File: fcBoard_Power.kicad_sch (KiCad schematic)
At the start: 24 parts, among them J1 DC_12V, U1 LM2596S-5, U2 LM2596S-ADJ, U3 LM2596S-ADJ

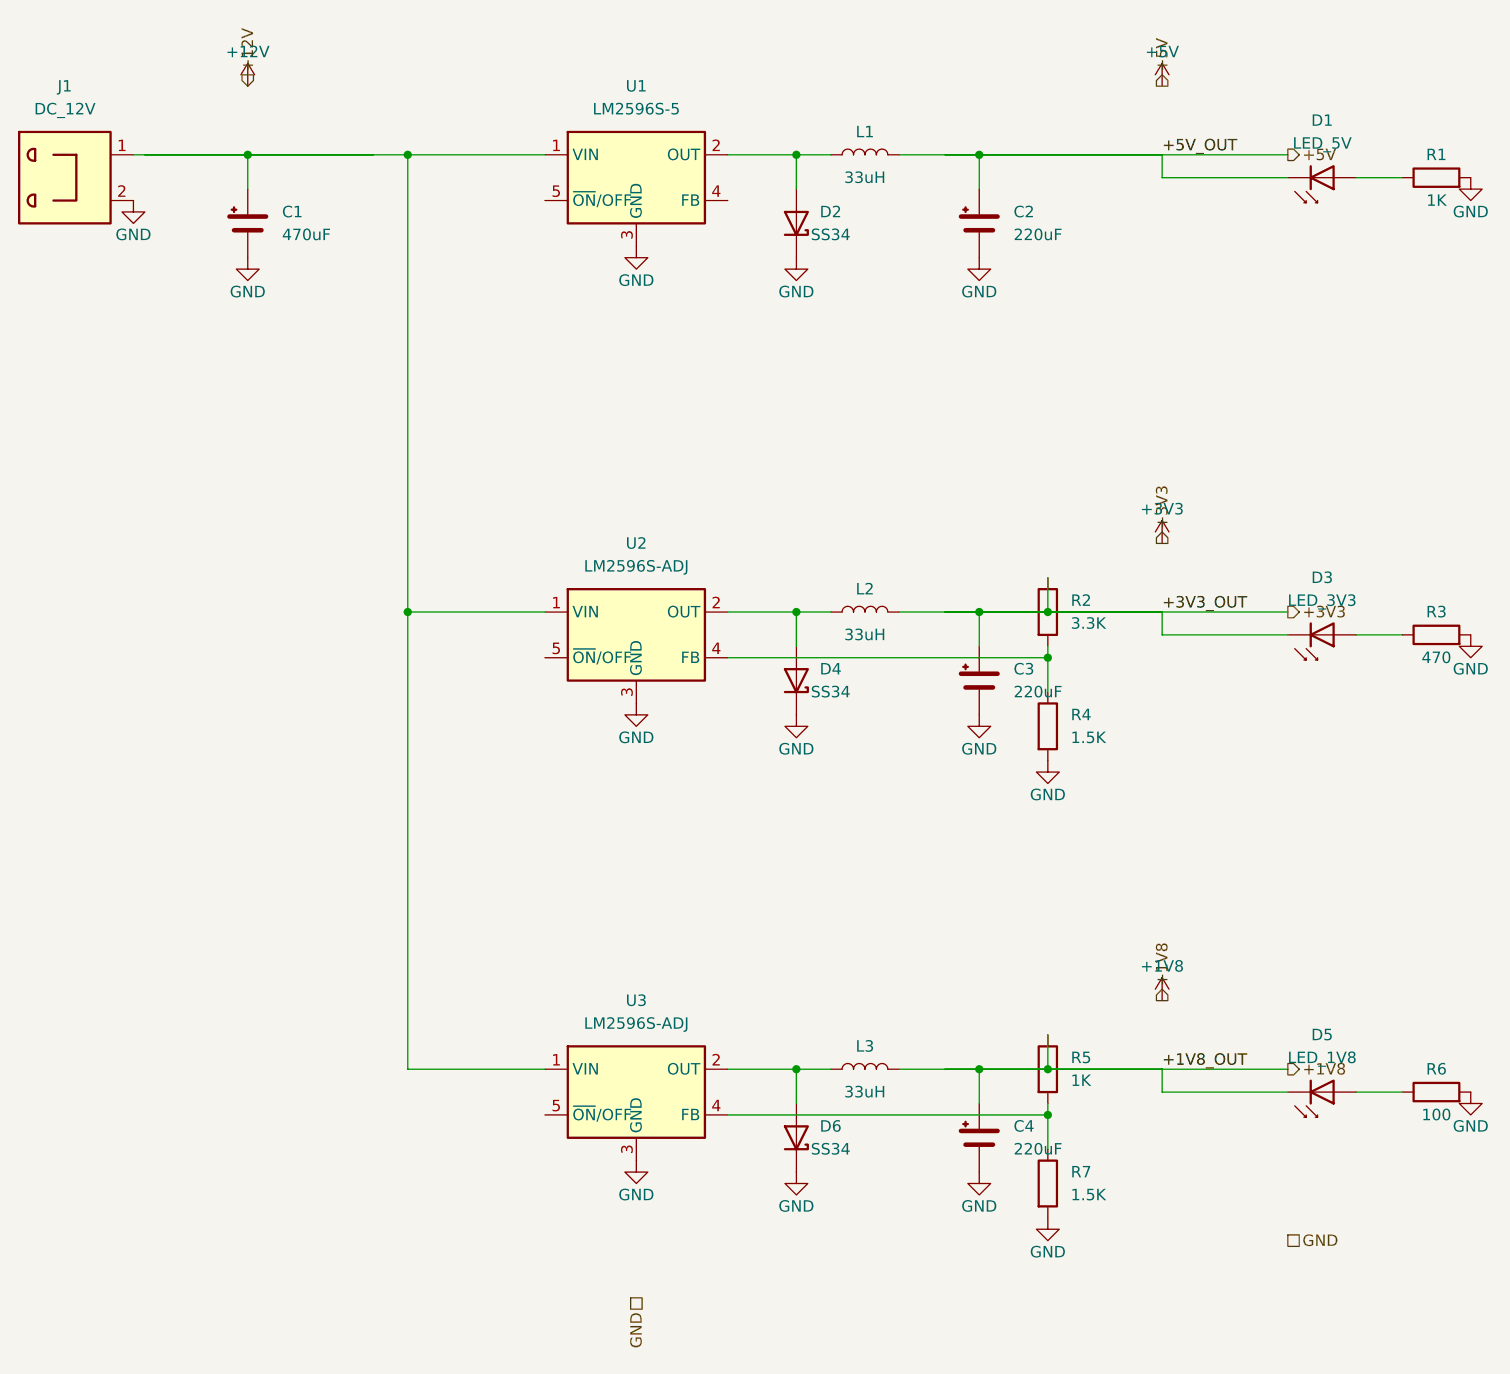
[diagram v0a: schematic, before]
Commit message: 회로도 라벨
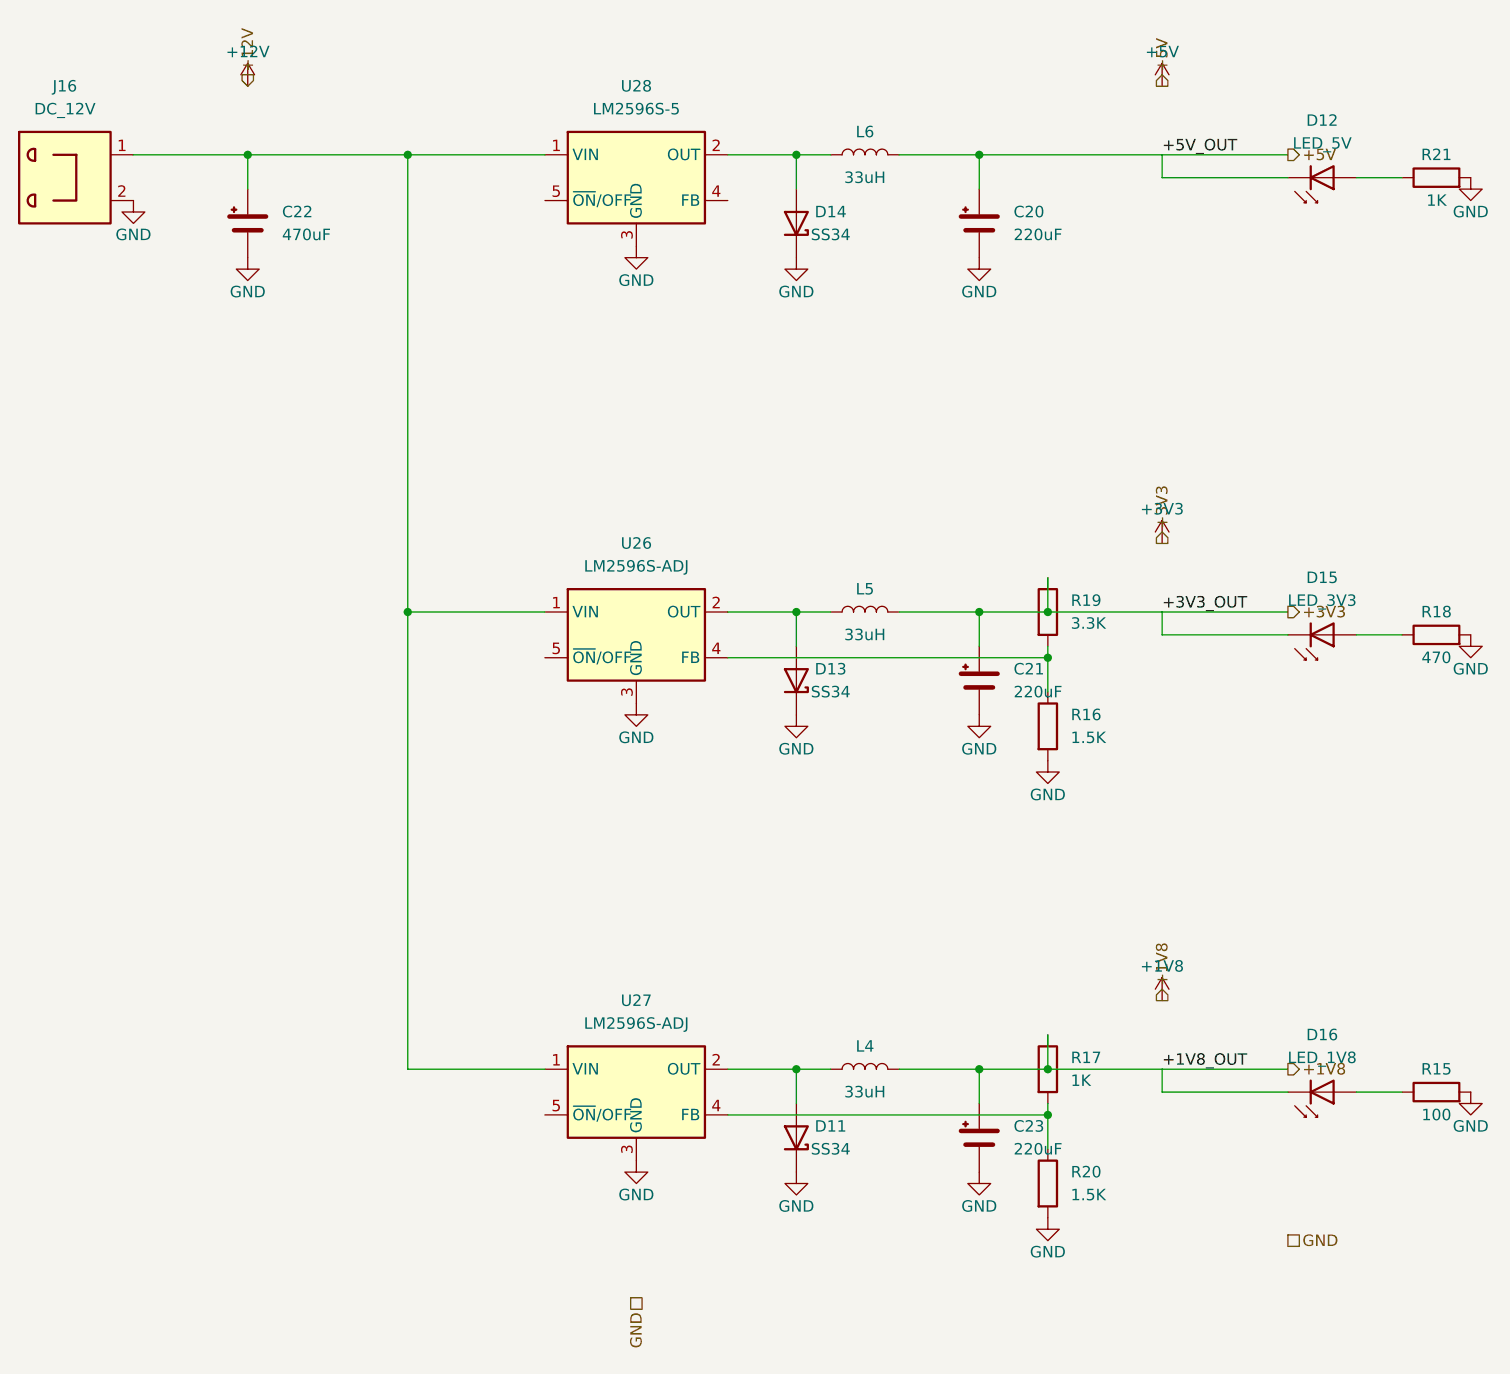
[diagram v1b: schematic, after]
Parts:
- renumbered C2 to C20, C3 to C21, C1 to C22, C4 to C23, D6 to D11, D1 to D12, D4 to D13, D2 to D14, D3 to D15, D5 to D16, J1 to J16, L3 to L4, L2 to L5, L1 to L6, R6 to R15, R4 to R16, R5 to R17, R3 to R18, R2 to R19, R7 to R20, R1 to R21, U2 to U26, U3 to U27, U1 to U28
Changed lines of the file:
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@@
 	(wire
 		(pts
-			(xy 219.71 130.81) (xy 227.33 130.81)
+			(xy 240.03 82.55) (xy 254 82.55)
 		)
 		(stroke
@@
 	(wire
 		(pts
-			(xy 240.03 82.55) (xy 254 82.55)
+			(xy 227.33 177.8) (xy 227.33 181.61)
 		)
 		(stroke
@@
 	(wire
 		(pts
-			(xy 227.33 177.8) (xy 227.33 181.61)
+			(xy 199.39 80.01) (xy 199.39 83.82)
 		)
 		(stroke
@@
 	(wire
 		(pts
-			(xy 199.39 80.01) (xy 199.39 83.82)
+			(xy 125.73 80.01) (xy 138.43 80.01)
 		)
 		(stroke
@@
 	(wire
 		(pts
-			(xy 125.73 80.01) (xy 138.43 80.01)
+			(xy 191.77 130.81) (xy 199.39 130.81)
 		)
 		(stroke
@@
 	(wire
 		(pts
-			(xy 191.77 130.81) (xy 199.39 130.81)
+			(xy 199.39 130.81) (xy 199.39 134.62)
 		)
 		(stroke
@@
 	(wire
 		(pts
-			(xy 199.39 130.81) (xy 199.39 134.62)
+			(xy 240.03 181.61) (xy 254 181.61)
 		)
 		(stroke
@@
 	(wire
 		(pts
+			(xy 219.71 130.81) (xy 227.33 130.81)
+		)
+		(stroke
+			(width 0)
+			(type default)
+		)
+	)
+	(wire
+		(pts
 			(xy 240.03 130.81) (xy 240.03 133.35)
 		)
@@
 	(wire
 		(pts
+			(xy 240.03 130.81) (xy 254 130.81)
+		)
+		(stroke
+			(width 0)
+			(type default)
+		)
+	)
+	(wire
+		(pts
 			(xy 219.71 130.81) (xy 219.71 134.62)
 		)
@@
 	(wire
 		(pts
+			(xy 240.03 80.01) (xy 254 80.01)
+		)
+		(stroke
+			(width 0)
+			(type default)
+		)
+	)
+	(wire
+		(pts
 			(xy 227.33 139.7) (xy 227.33 135.89)
 		)
@@
 		)
 	)
+	(hierarchical_label "+5V"
+		(shape output)
+		(at 254 80.01 0)
+		(effects
+			(font
+				(size 1.27 1.27)
+			)
+			(justify left)
+		)
+	)
+	(hierarchical_label "+3V3"
+		(shape output)
+		(at 254 130.81 0)
+		(effects
+			(font
+				(size 1.27 1.27)
+			)
+			(justify left)
+		)
+	)
 	(hierarchical_label "+3V3"
 		(shape output)
@@
 		)
 	)
+	(hierarchical_label "+1V8"
+		(shape output)
+		(at 254 181.61 0)
+		(effects
+			(font
+				(size 1.27 1.27)
+			)
+			(justify left)
+		)
+	)
 	(hierarchical_label "+12V"
 		(shape input)
@@
 	(hierarchical_label "GND"
 		(shape passive)
+		(at 254 200.66 0)
+		(effects
+			(font
+				(size 1.27 1.27)
+			)
+			(justify left)
+		)
+	)
+	(hierarchical_label "GND"
+		(shape passive)
 		(at 181.61 207.01 270)
 		(effects
@@
 		(on_board yes)
 		(dnp no)
-		(property "Reference" "R6"
+		(property "Reference" "R15"
 			(at 270.51 181.61 90)
 			(effects
@@
 		(on_board yes)
 		(dnp no)
-		(property "Reference" "D6"
+		(property "Reference" "D11"
 			(at 203.2 187.96 90)
 			(effects
@@
 		(on_board yes)
 		(dnp no)
-		(property "Reference" "J1"
+		(property "Reference" "J16"
 			(at 118.11 72.39 0)
 			(effects
@@
 		(on_board yes)
 		(dnp no)
-		(property "Reference" "L3"
+		(property "Reference" "L4"
 			(at 207.01 179.07 90)
 			(effects
@@
 		(on_board yes)
 		(dnp no)
-		(property "Reference" "C2"
+		(property "Reference" "C20"
 			(at 223.52 86.36 0)
 			(effects
@@
 		(on_board yes)
 		(dnp no)
-		(property "Reference" "C3"
+		(property "Reference" "C21"
 			(at 223.52 137.16 0)
 			(effects
@@
 		(on_board yes)
 		(dnp no)
-		(property "Reference" "R4"
+		(property "Reference" "R16"
 			(at 229.87 142.24 0)
 			(effects
@@
 		(on_board yes)
 		(dnp no)
-		(property "Reference" "R5"
+		(property "Reference" "R17"
 			(at 229.87 180.34 0)
 			(effects
@@
 		(on_board yes)
 		(dnp no)
-		(property "Reference" "D1"
+		(property "Reference" "D12"
 			(at 257.81 76.2 0)
 			(effects
@@
 		(on_board yes)
 		(dnp no)
-		(property "Reference" "U2"
+		(property "Reference" "U26"
 			(at 181.61 123.19 0)
 			(effects
@@
 		(on_board yes)
 		(dnp no)
-		(property "Reference" "R3"
+		(property "Reference" "R18"
 			(at 270.51 130.81 90)
 			(effects
@@
 		(on_board yes)
 		(dnp no)
-		(property "Reference" "L2"
+		(property "Reference" "L5"
 			(at 207.01 128.27 90)
 			(effects
@@
 		(on_board yes)
 		(dnp no)
-		(property "Reference" "D4"
+		(property "Reference" "D13"
 			(at 203.2 137.16 90)
 			(effects
@@
 		(on_board yes)
 		(dnp no)
-		(property "Reference" "R2"
+		(property "Reference" "R19"
 			(at 229.87 129.54 0)
 			(effects
@@
 		(on_board yes)
 		(dnp no)
-		(property "Reference" "C1"
+		(property "Reference" "C22"
 			(at 142.24 86.36 0)
 			(effects
@@
 		(on_board yes)
 		(dnp no)
-		(property "Reference" "R7"
+		(property "Reference" "R20"
 			(at 229.87 193.04 0)
 			(effects
@@
 		(on_board yes)
 		(dnp no)
-		(property "Reference" "C4"
+		(property "Reference" "C23"
 			(at 223.52 187.96 0)
 			(effects
@@
 		(on_board yes)
 		(dnp no)
-		(property "Reference" "D2"
+		(property "Reference" "D14"
 			(at 203.2 86.36 90)
 			(effects
@@
 		(on_board yes)
 		(dnp no)
-		(property "Reference" "D3"
+		(property "Reference" "D15"
 			(at 257.81 127 0)
 			(effects
@@
 		(on_board yes)
 		(dnp no)
-		(property "Reference" "L1"
+		(property "Reference" "L6"
 			(at 207.01 77.47 90)
 			(effects
@@
 		(on_board yes)
 		(dnp no)
-		(property "Reference" "U3"
+		(property "Reference" "U27"
 			(at 181.61 173.99 0)
 			(effects
@@
 		(on_board yes)
 		(dnp no)
-		(property "Reference" "D5"
+		(property "Reference" "D16"
 			(at 257.81 177.8 0)
 			(effects
@@
 		(on_board yes)
 		(dnp no)
-		(property "Reference" "R1"
+		(property "Reference" "R21"
 			(at 270.51 80.01 90)
 			(effects
@@
 		(on_board yes)
 		(dnp no)
-		(property "Reference" "U1"
+		(property "Reference" "U28"
 			(at 181.61 72.39 0)
 			(effects
@@
 		)
 	)
-	(wire
-		(pts
-			(xy 127.0 80.01)
-			(xy 152.4 80.01)
-		)
-		(stroke
-			(width 0)
-			(type default)
-		)
-	)
-	(wire
-		(pts
-			(xy 215.9 80.01)
-			(xy 240.03 80.01)
-		)
-		(stroke
-			(width 0)
-			(type default)
-		)
-	)
-	(wire
-		(pts
-			(xy 215.9 130.81)
-			(xy 240.03 130.81)
-		)
-		(stroke
-			(width 0)
-			(type default)
-		)
-	)
-	(wire
-		(pts
-			(xy 215.9 181.61)
-			(xy 240.03 181.61)
-		)
-		(stroke
-			(width 0)
-			(type default)
-		)
-	)
-	(wire
-		(pts
-			(xy 240.03 80.01)
-			(xy 254.0 80.01)
-		)
-		(stroke
-			(width 0)
-			(type default)
-		)
-	)
-	(wire
-		(pts
-			(xy 240.03 130.81)
-			(xy 254.0 130.81)
-		)
-		(stroke
-			(width 0)
-			(type default)
-		)
-	)
-	(wire
-		(pts
-			(xy 240.03 181.61)
-			(xy 254.0 181.61)
-		)
-		(stroke
-			(width 0)
-			(type default)
-		)
-	)
-	(hierarchical_label "+5V"
-		(shape output)
-		(at 254.0 80.01 0)
-		(fields_autoplaced yes)
-		(effects
-			(font
-				(size 1.27 1.27)
-			)
-			(justify left)
-		)
-	)
-	(hierarchical_label "+3V3"
-		(shape output)
-		(at 254.0 130.81 0)
-		(fields_autoplaced yes)
-		(effects
-			(font
-				(size 1.27 1.27)
-			)
-			(justify left)
-		)
-	)
-	(hierarchical_label "+1V8"
-		(shape output)
-		(at 254.0 181.61 0)
-		(fields_autoplaced yes)
-		(effects
-			(font
-				(size 1.27 1.27)
-			)
-			(justify left)
-		)
-	)
-	(hierarchical_label "GND"
-		(shape passive)
-		(at 254.0 200.66 0)
-		(fields_autoplaced yes)
-		(effects
-			(font
-				(size 1.27 1.27)
-			)
-			(justify left)
-		)
-	))
+)
